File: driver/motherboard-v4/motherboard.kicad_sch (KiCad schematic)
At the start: 1 part

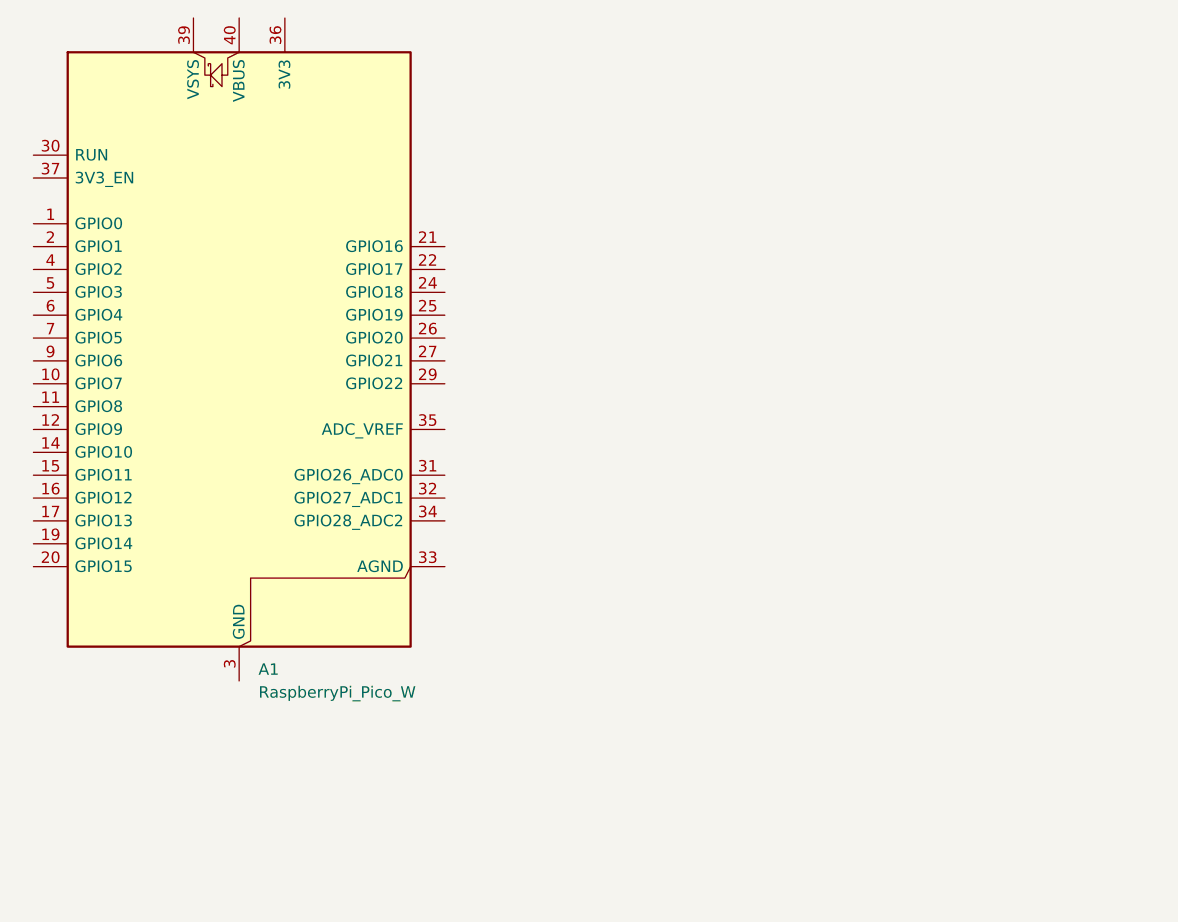
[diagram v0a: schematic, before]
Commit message: Add motherboard fritzing.
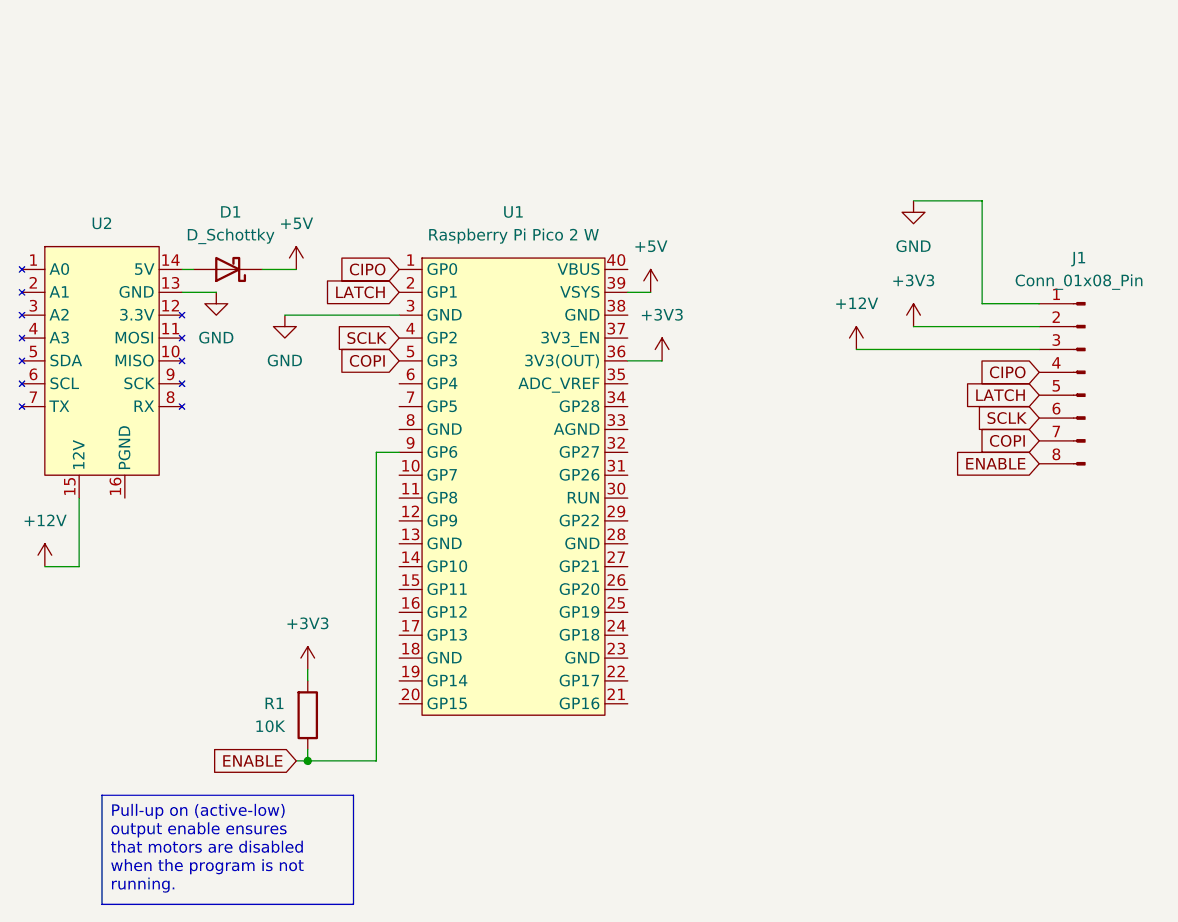
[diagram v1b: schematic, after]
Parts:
- removed A1: RaspberryPi_Pico_W, Module:RaspberryPi_Pico_W_SMD, symbol MCU_Module:RaspberryPi_Pico_W
- added D1: D_Schottky, Diode_THT:D_5W_P10.16mm_Horizontal, symbol Device:D_Schottky
- added J1: Conn_01x08_Pin, Connector:Tag-Connect_TC2030-IDC-FP_2x03_P1.27mm_Vertical, symbol Connector:Conn_01x08_Pin
- added R1: 10K, Package_QFP:LQFP-32_7x7mm_P0.8mm, symbol Device:R
- added U1: Raspberry Pi Pico 2 W, Module:RaspberryPi_Pico_W_SMD, symbol MCU_Module:RaspberryPi_Pico_W_Physical
- added U2: (no value), custom:adafruit BFF, symbol custom:Adafruit_DC_Power_BFF
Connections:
- new net: D1.2 (A), U2.14 (5V)
- new net +12V: J1.3 (Pin_3), U2.15 (12V)
- new net +3V3: J1.2 (Pin_2), R1.2, U1.36 (3V3(OUT))
- new net +5V: D1.1 (K), U1.39 (VSYS)
- new net CIPO: J1.4 (Pin_4), U1.1 (GP0)
- new net COPI: J1.7 (Pin_7), U1.5 (GP3)
- new net ENABLE: J1.8 (Pin_8), R1.1, U1.9 (GP6)
- new net GND: J1.1 (Pin_1), U1.3 (GND), U2.13 (GND)
- new net LATCH: J1.5 (Pin_5), U1.2 (GP1)
- new net SCLK: J1.6 (Pin_6), U1.4 (GP2)
